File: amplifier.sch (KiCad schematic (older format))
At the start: 0 parts

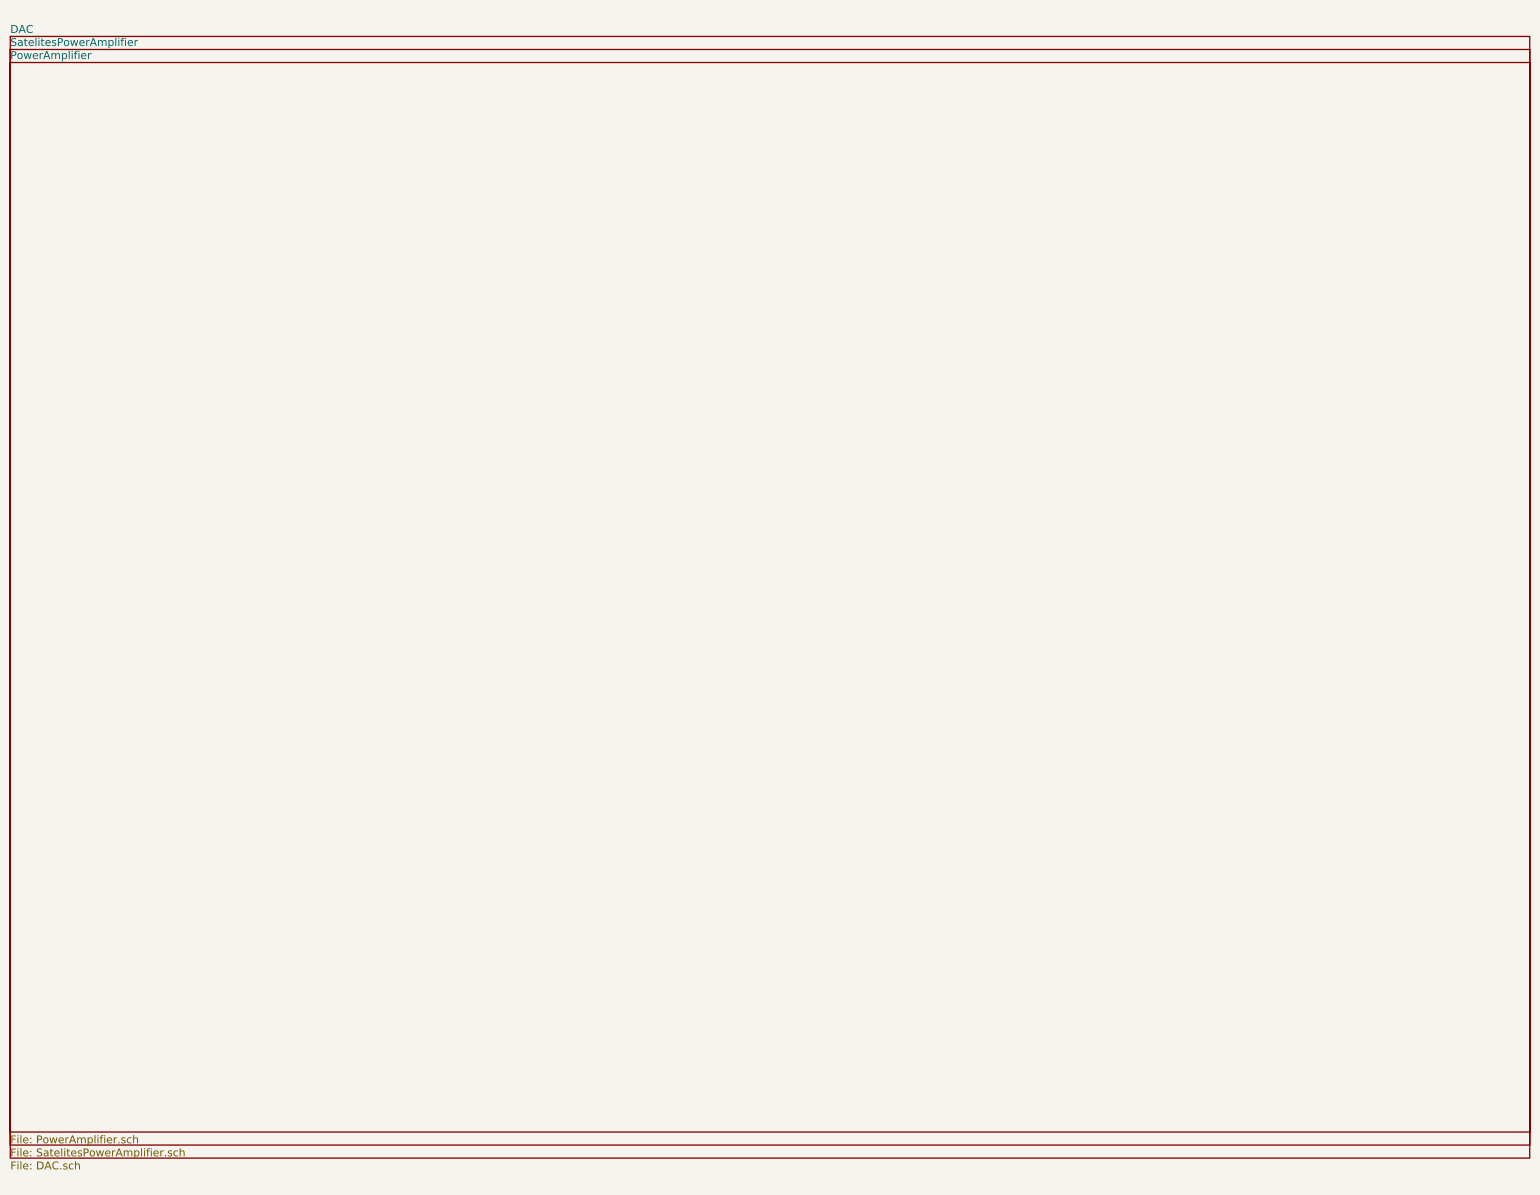
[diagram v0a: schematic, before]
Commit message: Update DAC
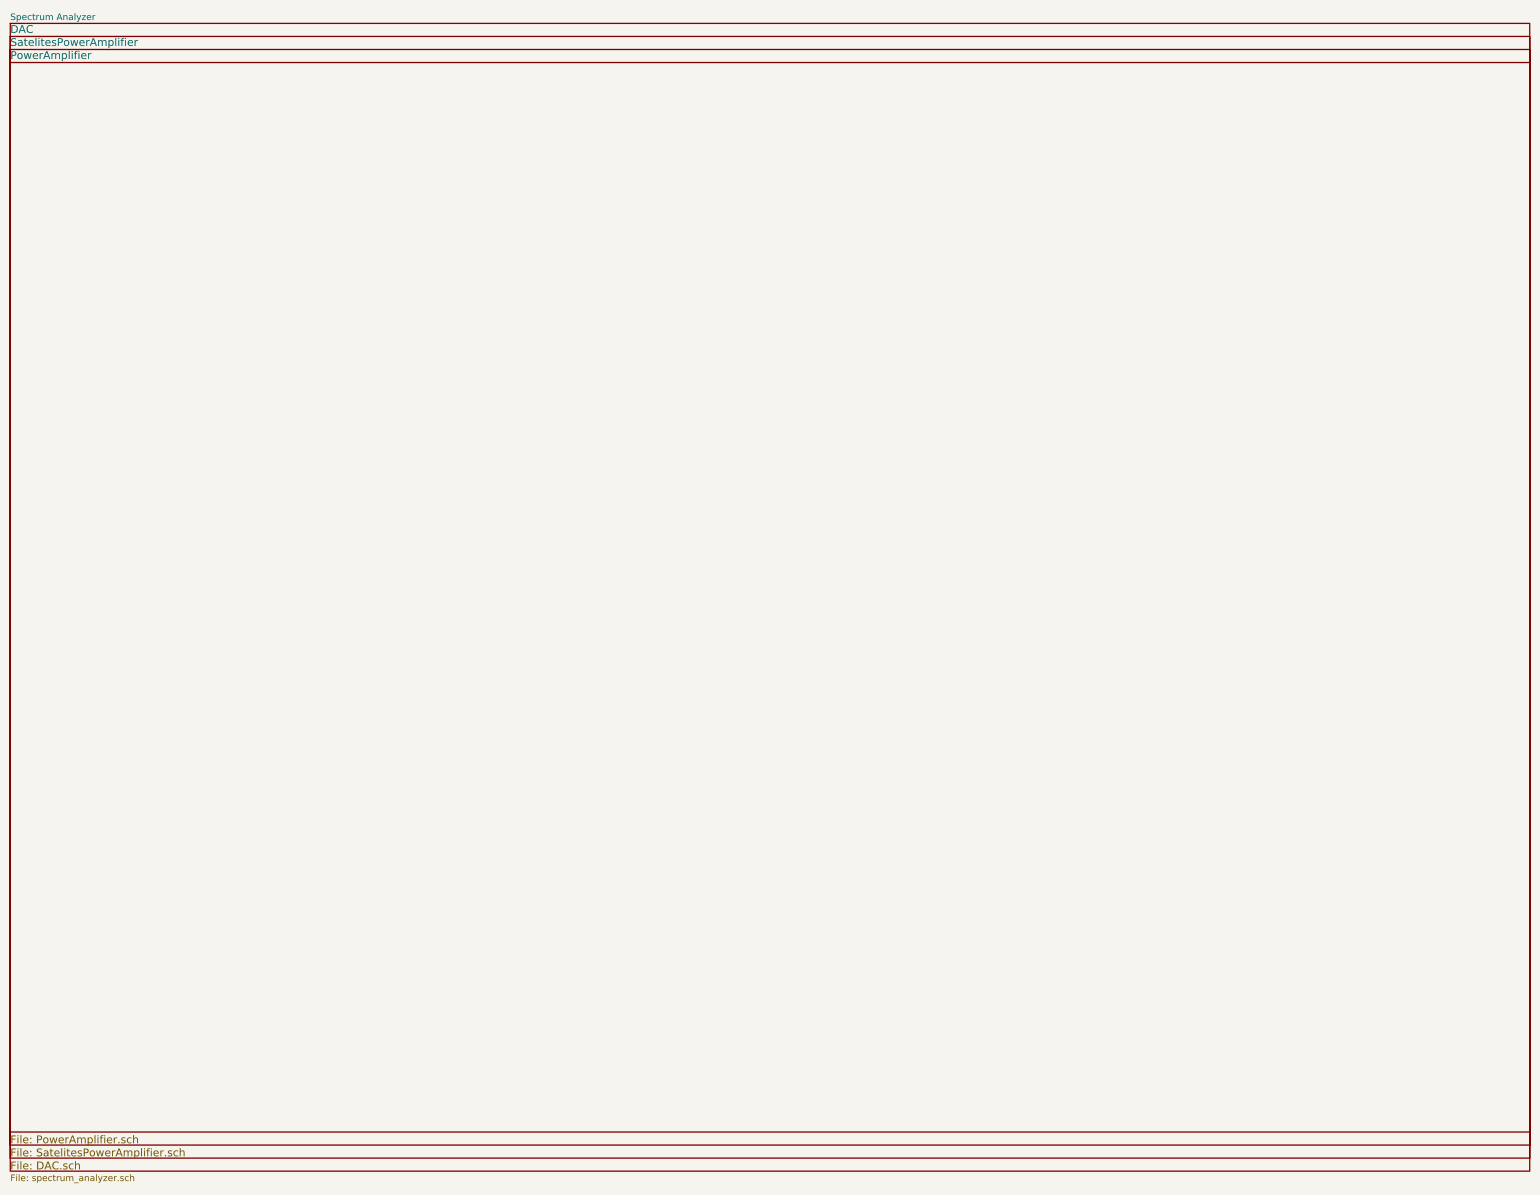
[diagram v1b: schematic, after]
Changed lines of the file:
@@
-EESchema Schematic File Version 2
-LIBS:amplifier-rescue
-LIBS:ad1955
-LIBS:cdclvc1104
-LIBS:kc7050
-LIBS:lp5900
-LIBS:src4392i
-LIBS:tda7293v
-LIBS:74xgxx
-LIBS:74xx
-LIBS:ac-dc
-LIBS:adc-dac
-LIBS:analog_switches
-LIBS:atmel
-LIBS:audio
-LIBS:brooktre
-LIBS:cmos4000
-LIBS:cmos_ieee
-LIBS:conn
-LIBS:contrib
-LIBS:cypress
-LIBS:dc-dc
-LIBS:device
-LIBS:digital-audio
-LIBS:display
-LIBS:dsp
-LIBS:elec-unifil
-LIBS:ftdi
-LIBS:gennum
-LIBS:graphic
-LIBS:hc11
-LIBS:intel
-LIBS:interface
-LIBS:linear
-LIBS:logo
-LIBS:memory
-LIBS:microchip
-LIBS:microchip1
-LIBS:microchip_pic10mcu
-LIBS:microchip_pic12mcu
-LIBS:microchip_pic16mcu
-LIBS:microcontrollers
-LIBS:motorola
-LIBS:msp430
-LIBS:nxp_armmcu
-LIBS:opto
-LIBS:philips
-LIBS:power
-LIBS:powerint
-LIBS:pspice
-LIBS:references
-LIBS:regul
-LIBS:relays
-LIBS:sensors
-LIBS:siliconi
-LIBS:special
-LIBS:stm8
-LIBS:stm32
-LIBS:supertex
-LIBS:texas
-LIBS:transf
-LIBS:transistors
-LIBS:ttl_ieee
-LIBS:valves
-LIBS:video
-LIBS:xilinx
-LIBS:ad8066
-LIBS:ldk220
-LIBS:+9va
+EESchema Schematic File Version 4
 LIBS:amplifier-cache
-EELAYER 25 0
+EELAYER 26 0
 EELAYER END
 $Descr A4 11693 8268
 encoding utf-8
-Sheet 1 4
+Sheet 1 5
 Title ""
 Date ""
@@
 F1 "PowerAmplifier.sch" 60
 $EndSheet
+$Sheet
+S 0    -300 11650 8800
+U 5C997C50
+F0 "Spectrum Analyzer" 50
+F1 "spectrum_analyzer.sch" 50
+$EndSheet
 $EndSCHEMATC
